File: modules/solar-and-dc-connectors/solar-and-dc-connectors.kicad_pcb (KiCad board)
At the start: 2 copper layers, 19.3 x 32.1 mm, 3 parts, among them J1 S2B-PH-K-SLFSN, J2 54-00127

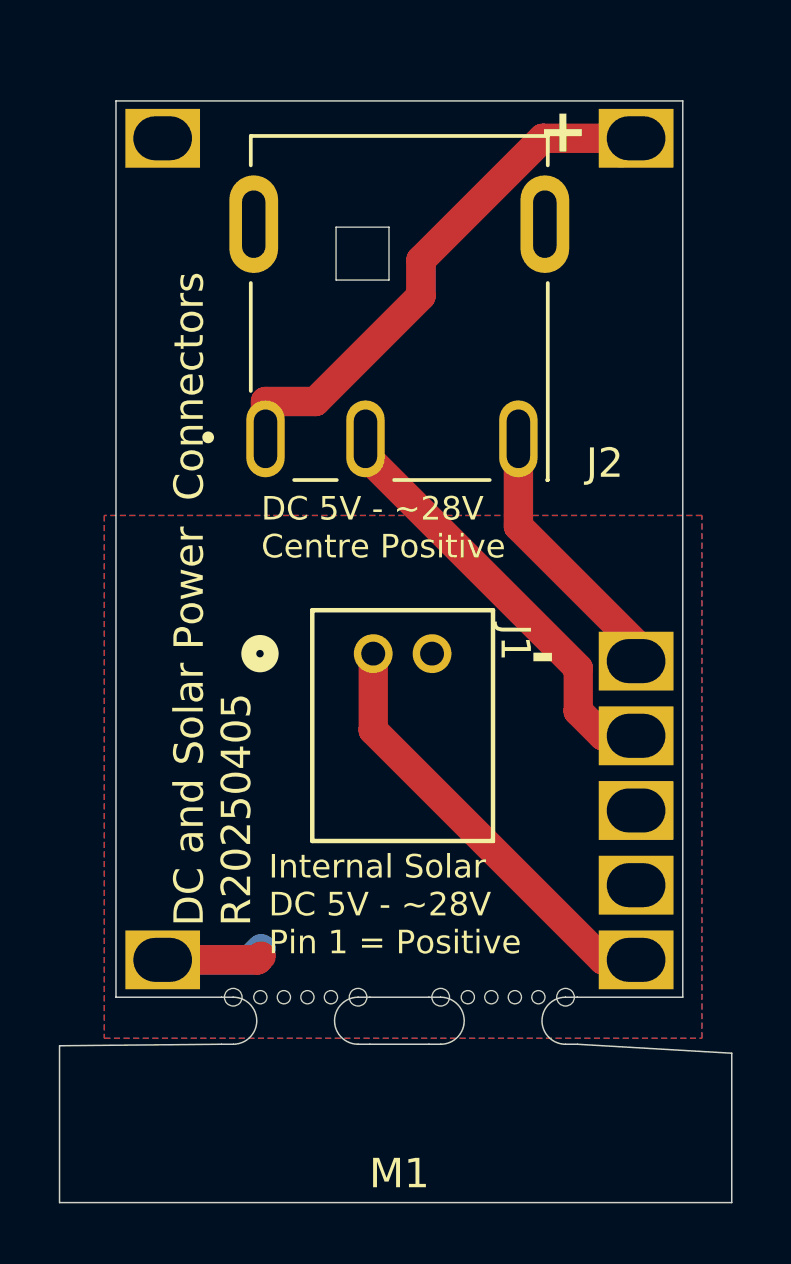
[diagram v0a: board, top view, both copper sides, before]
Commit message: Updating solar-and-dc
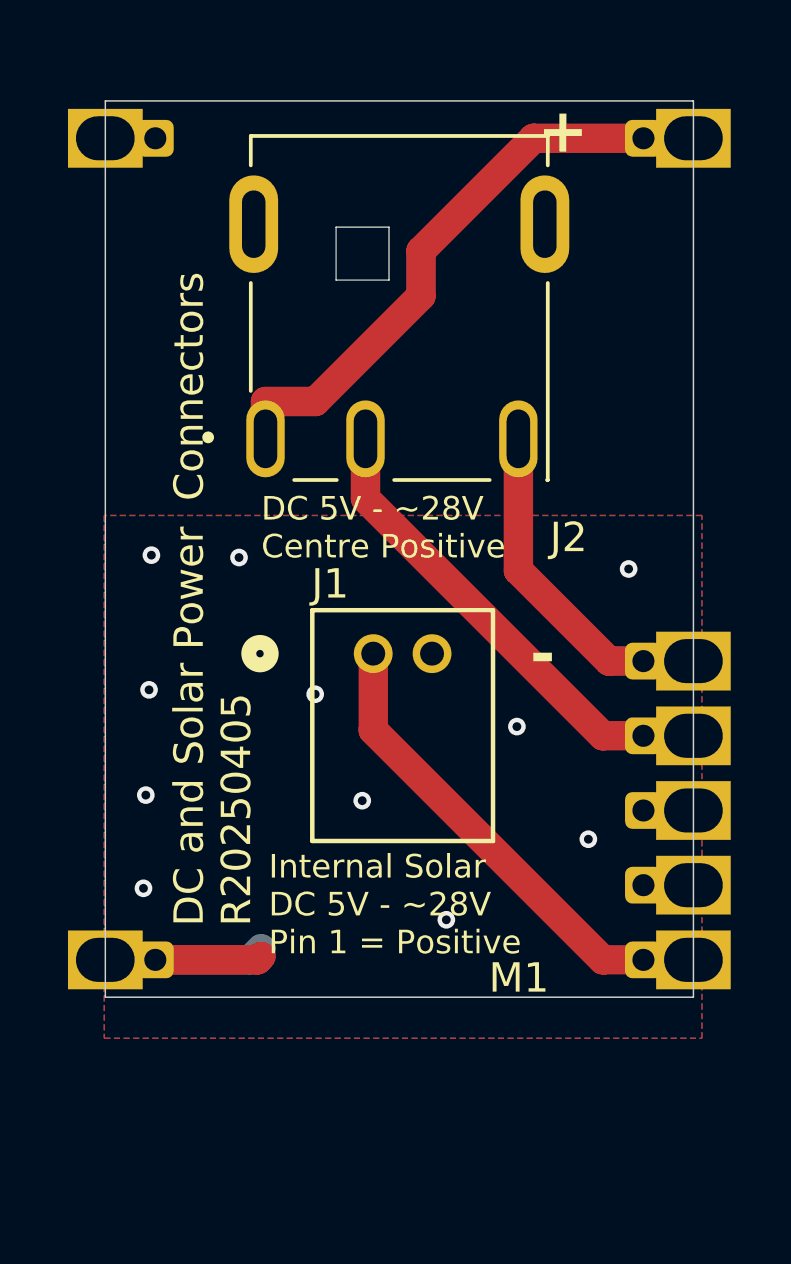
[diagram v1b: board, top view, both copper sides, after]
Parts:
- J1: footprint footprints:CONN_S2B-PH-K-S_JST -> MegaCastle:CONN_S2B-PH-K-S_JST
- J2: footprint footprints:TENSILITY_54-00127 -> MegaCastle:TENSILITY_54-00127
- M1: footprint MegaCastle:MegaCastle2x12-Module-I12.5x25.7-M80181F-PANEL-NIBBLE -> MegaCastle:MegaCastle2x12-Module-I20.0x25.7-M80181F-SPAREPAD
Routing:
- net DIRTY_DC_-: track 9.22 -> 9.76 mm
- net DIRTY_DC_+: track 19.0 -> 18.5 mm
- net GND: vias 0 -> 11
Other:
- board size 19.3 x 32.1 mm -> 20 x 30.5 mm
